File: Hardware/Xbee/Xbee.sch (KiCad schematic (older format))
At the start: 39 parts, among them J1 Alimentación, J2 Raspberry, J3 Pines 1, J4 Pines 2, J5 Programación, J6 Entrada, J7 Salida, K1 SANYOU_SRD_Form_C, Q1 2N7002, Q2 AP2300, SW1 Reset, SW2 Comm., U1 AZ1117-3.3, U2 Xbee, U3 LM358

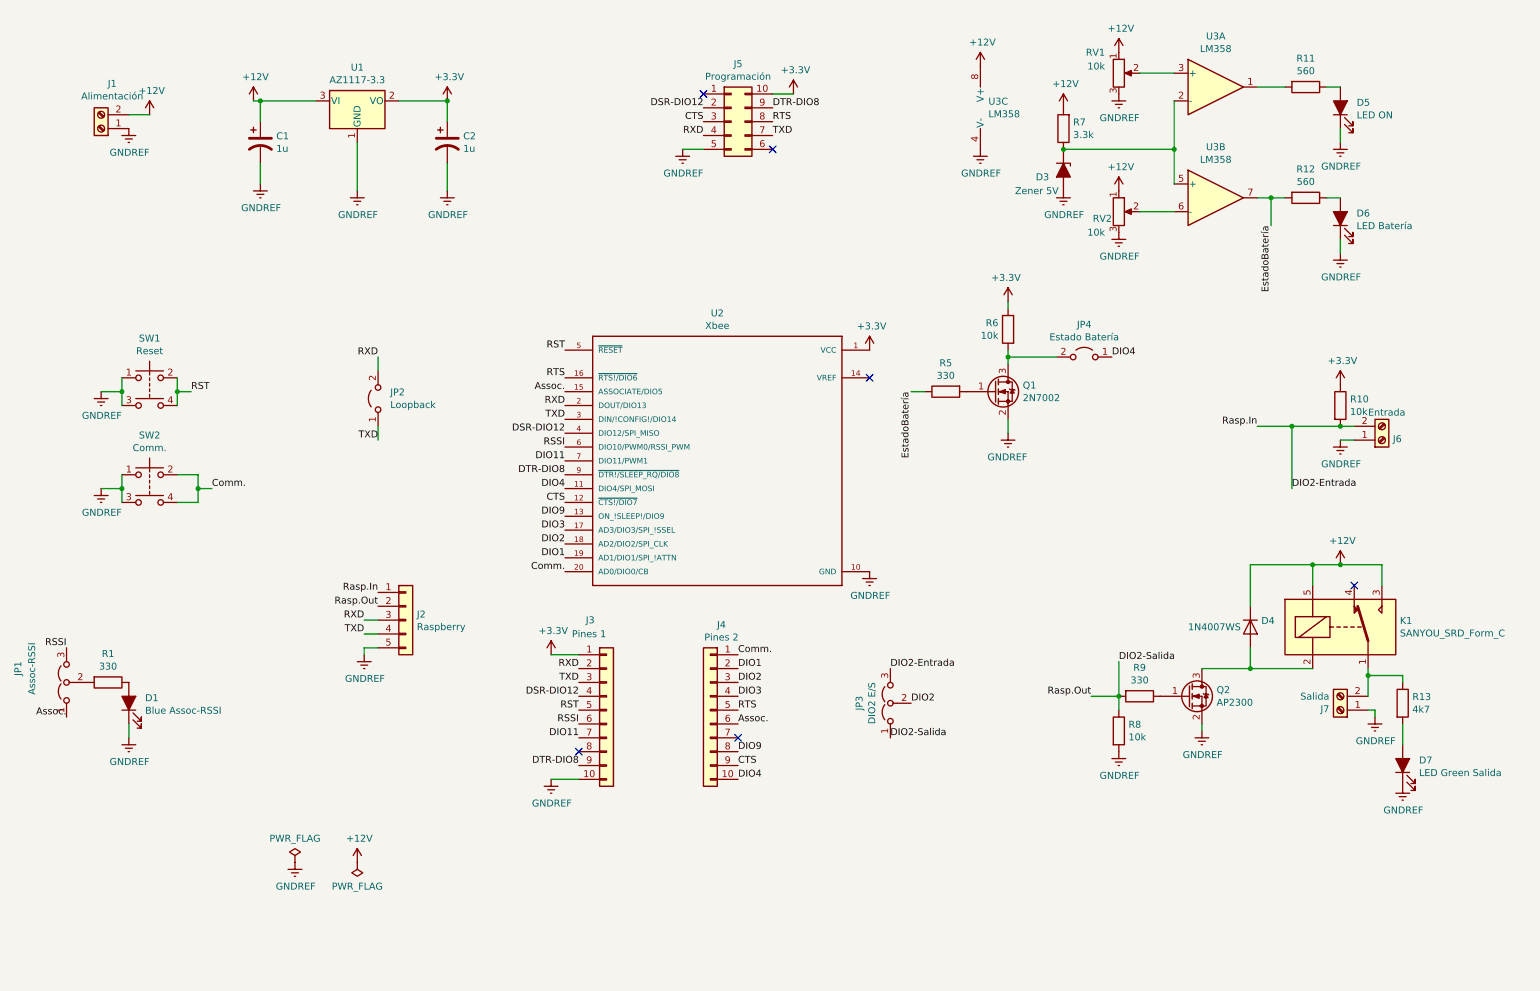
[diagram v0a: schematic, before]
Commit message: Sheets-Text
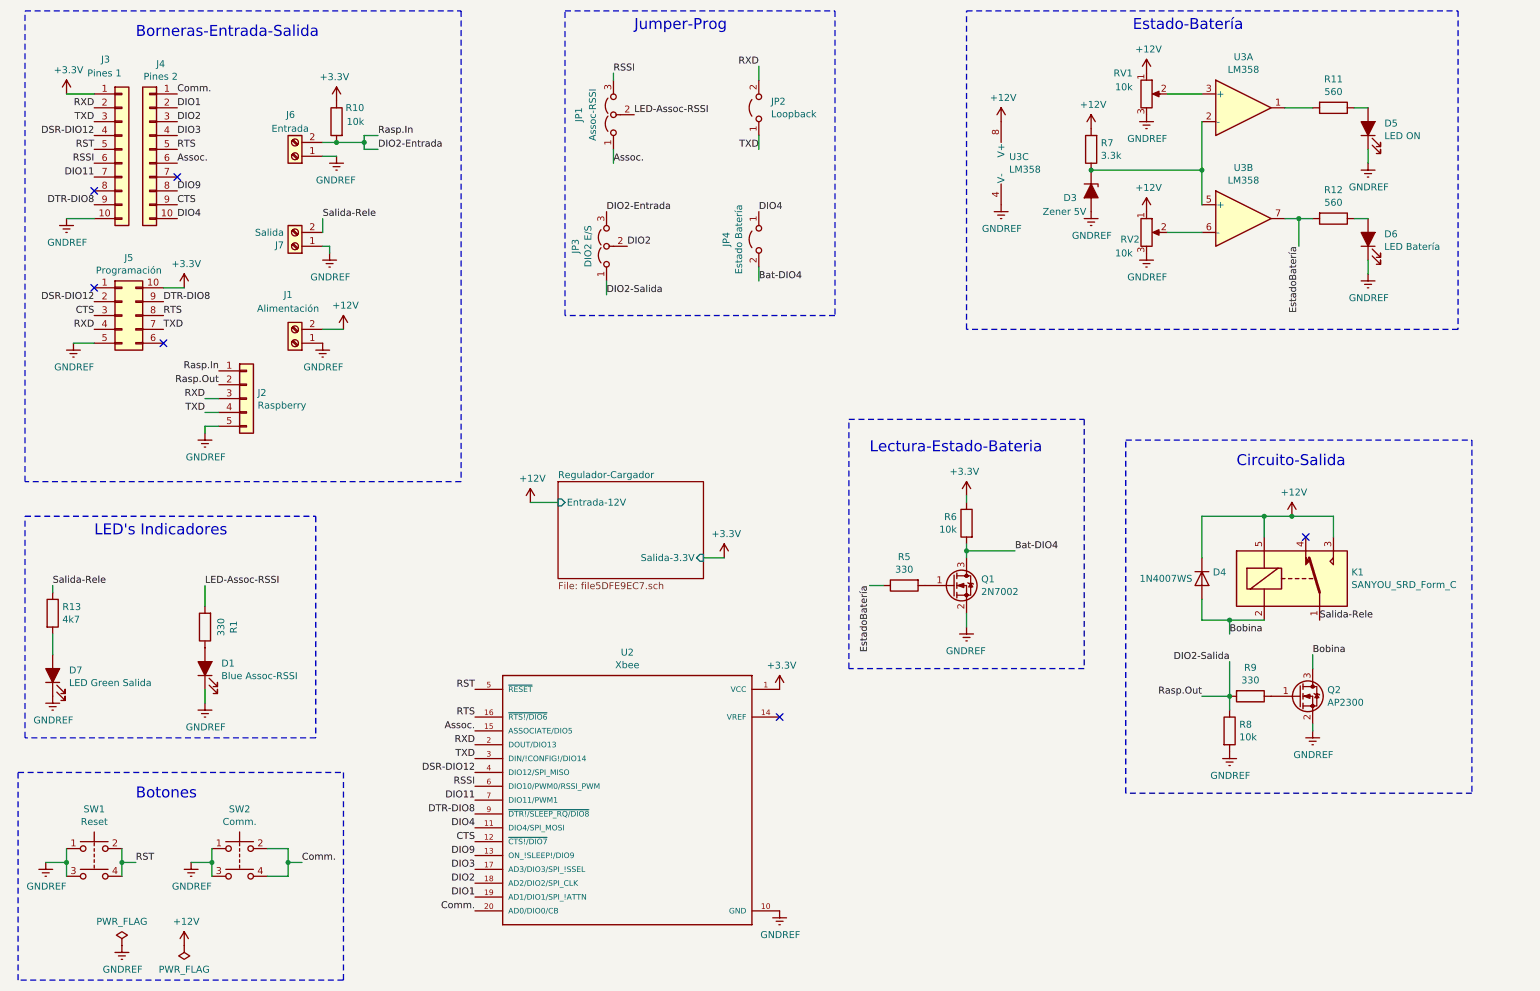
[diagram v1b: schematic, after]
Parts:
- removed C1, C2: 1u, Capacitor_SMD:C_0805_2012Metric, symbol Xbee-rescue:CP1-Device
- removed U1: AZ1117-3.3, Package_TO_SOT_SMD:SOT-223-3_TabPin2, symbol Regulator_Linear:AZ1117-3.3
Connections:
- net LED-Assoc-RSSI: now reaches JP1.2 (C), R1.2
- net Bobina: now reaches D4.2 (A), K1.2, Q2.3 (D)
- net Salida-Rele: now reaches J7.2 (Pin_2), K1.1, R13.1
- net Bat-DIO4: now reaches JP4.2 (B), Q1.3 (D), R6.2
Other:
- note added: "Borneras-Entrada-Salida"
- note added: "Botones"
- note added: "Circuito-Salida"
- note added: "Estado-Batería"
- note added: "Jumper-Prog"
- note added: "LED's Indicadores"
- note added: "Lectura-Estado-Bateria"
- moved on the sheet: D1, D3, D4, D5, D6, D7, J1, J2, J3, J4, J5, J6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
